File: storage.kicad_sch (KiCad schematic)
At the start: 27 parts, among them J4 uSD card, J5 uSD card, P1 uBUS1, P2 uBUS2, P3 uBUS3, Q1 BC856, Q2 BC856, U10 IS61WV20488BLL-10TLI, U11 MT48LC16M16A2TG, U9 IS61WV20488BLL-10TLI

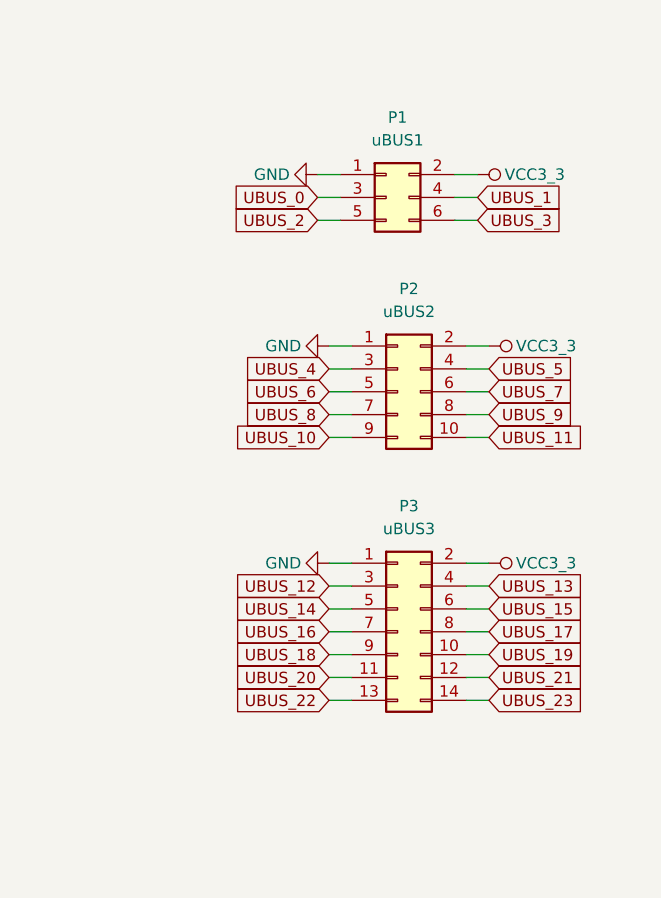
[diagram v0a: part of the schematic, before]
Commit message: revG
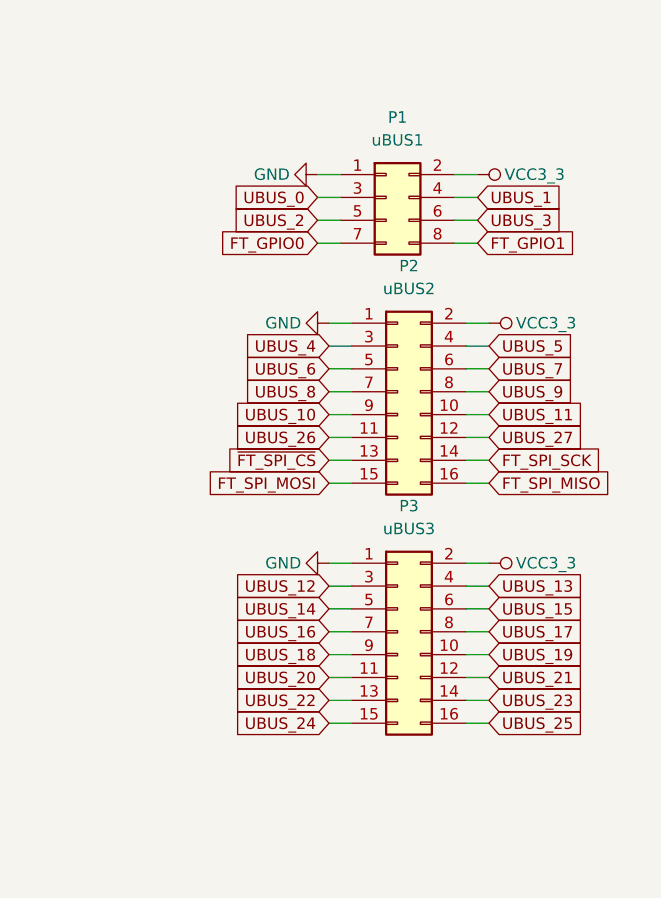
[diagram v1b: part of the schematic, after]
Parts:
- P1: footprint Connector_PinHeader_1.27mm:PinHeader_2x03_P1.27mm_Vertical -> Connector_PinHeader_1.27mm:PinHeader_2x04_P1.27mm_Vertical; symbol Connector_Generic:Conn_02x03_Odd_Even -> Connector_Generic:Conn_02x04_Odd_Even
- P2: footprint Connector_PinHeader_1.27mm:PinHeader_2x05_P1.27mm_Vertical -> Connector_PinHeader_1.27mm:PinHeader_2x08_P1.27mm_Vertical; symbol Connector_Generic:Conn_02x05_Odd_Even -> Connector_Generic:Conn_02x08_Odd_Even
- P3: footprint Connector_PinHeader_1.27mm:PinHeader_2x07_P1.27mm_Vertical -> Connector_PinHeader_1.27mm:PinHeader_2x08_P1.27mm_Vertical; symbol Connector_Generic:Conn_02x07_Odd_Even -> Connector_Generic:Conn_02x08_Odd_Even
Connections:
- new net FT_GPIO0: P1.7 (Pin_7)
- new net FT_GPIO1: P1.8 (Pin_8)
- new net FT_SPI_MISO: P2.16 (Pin_16)
- new net FT_SPI_MOSI: P2.15 (Pin_15)
- new net FT_SPI_SCK: P2.14 (Pin_14)
- new net UBUS_24: P3.15 (Pin_15)
- new net UBUS_25: P3.16 (Pin_16)
- new net UBUS_26: P2.11 (Pin_11)
- new net UBUS_27: P2.12 (Pin_12)
- new net ~{FT_SPI_CS}: P2.13 (Pin_13)
